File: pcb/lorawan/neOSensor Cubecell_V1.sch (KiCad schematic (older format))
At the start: 22 parts, among them J1 Conn_01x05, J2 Conn_01x05, J3 Conn_01x04, J5 Conn_01x05, J6 Conn_01x04, J7 ATECC508A, SW1 G71Y, U1 HTCC-AB01, U2 HC-SR01, U3 OLED1.3_I2C

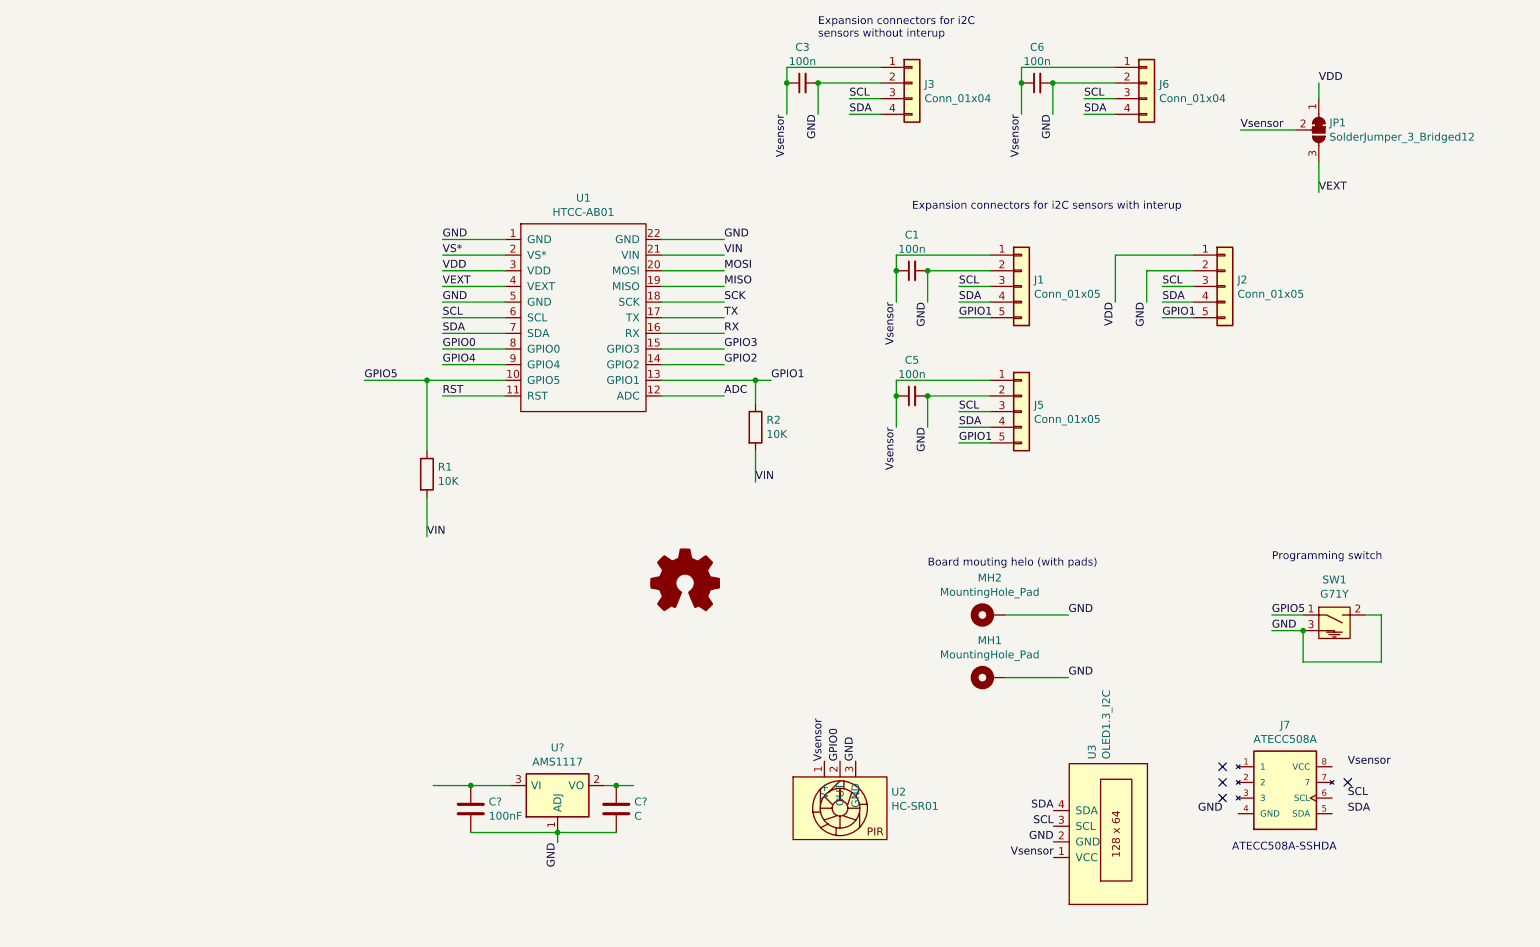
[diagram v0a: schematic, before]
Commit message: mise a jour des schema
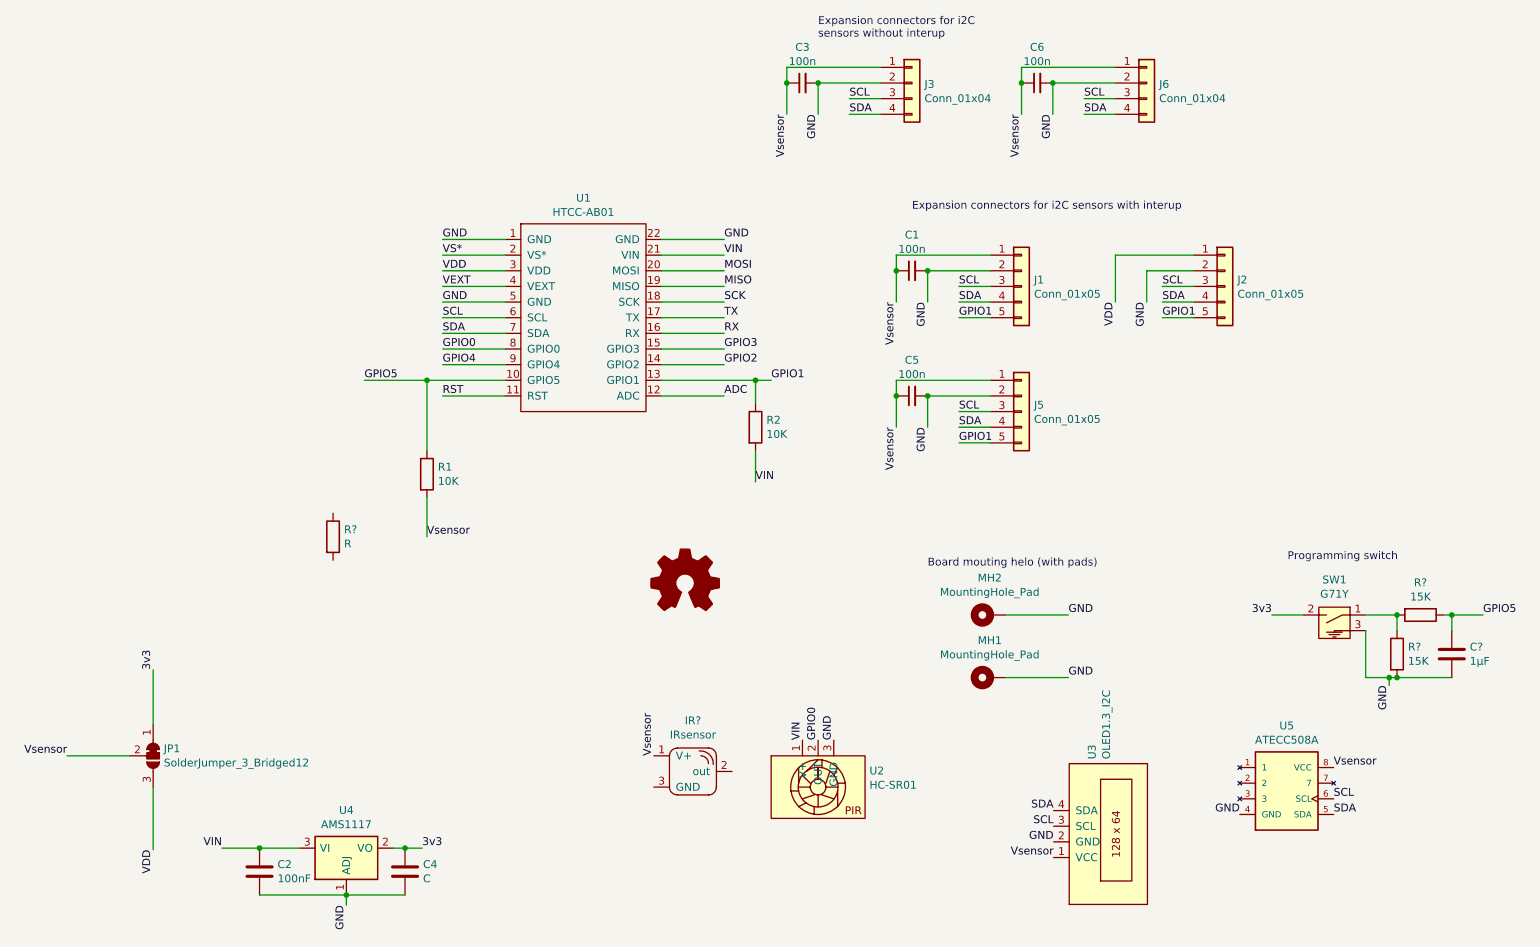
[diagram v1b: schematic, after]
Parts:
- removed J7: ATECC508A, neosensor_addon:ATECC508A, symbol neosensor_addon:ATECC508A
- removed SW1: G71Y, neosensor_addon:G71Y_µsw_smd, symbol neOSensor-Cubecell_V1-rescue:G71Y-neosensor_addon-neOSensor_Cubecell_V1-rescue
- removed U1: HTCC-AB01, HTCC-AB01:htcc-ab01, symbol neOSensor-Cubecell_V1-rescue:HTCC-AB01-htcc-ab01-neOSensor_Cubecell_V1-rescue
- added C?: 1µF, symbol Device:C
- added IR?: IRsensor, neosensor_addon:IRsensor_TH_and_smd, symbol neosensor_addon:IRsensor
- added R? (x2): 15K, symbol Device:R
- added R?: R, symbol Device:R
- added SW1: G71Y, neosensor_addon:G71Y_µsw_smd, symbol neosensor_addon:G71Y
- added U1: HTCC-AB01, neosensor_addon:HTCC-AB01, symbol neosensor_addon:HTCC-AB01
- added U5: ATECC508A, neosensor_addon:SOIC-8_3.9x5.4mm_P1.27mm_HandSolder, symbol neosensor_addon:ATECC508A
- C2, C4: renamed from C?; footprint (none) -> Capacitor_SMD:C_0805_2012Metric_Pad1.15x1.40mm_HandSolder
- gave numbers to parts that had none: 1
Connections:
- net ADC: now also U1.12 (ADC)
- net GND: now also C?.2, R?.2, SW1.3, U1.1 (GND), U1.22 (GND), U1.5 (GND), U5.4 (GND)
- net GPIO0: now also U1.8 (GPIO0)
- net GPIO1: now also U1.13 (GPIO1)
- net GPIO2: now also U1.14 (GPIO2)
- net GPIO3: now also U1.15 (GPIO3)
- net GPIO4: now also U1.9 (GPIO4)
- net GPIO5: now also C?.1, R?.1, U1.10 (GPIO5)
- net MISO: now also U1.19 (MISO)
- net MOSI: now also U1.20 (MOSI)
- net RST: now also U1.11 (RST)
- net RX: now also U1.16 (RX)
- net SCK: now also U1.18 (SCK)
- net SCL: now also U1.6 (SCL), U5.6 (SCL)
- net SDA: now also U1.7 (SDA), U5.5 (SDA)
- net TX: now also U1.17 (TX)
- net VDD: now also JP1.3 (B), U1.3 (VDD); no longer JP1.1 (A)
- net VEXT: now also U1.4 (VEXT); no longer JP1.3 (B)
- net VIN: now also C2.1, U2.1 (V+), U4.3 (VI), U1.21 (VIN); no longer R1.2
- net VS*: now also U1.2 (VS*)
- net Vsensor: now also R1.2, IR?.1 (V+), U5.8 (VCC); no longer U2.1 (V+)
- net 3v3: now reaches C4.1, U4.2 (VO)
- net 3v3: now also JP1.1 (A), SW1.2
- new net: R?.1, R?.2, SW1.1
- no-connect marks 4 -> 0
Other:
- note removed: "ATECC508A-SSHDA"
- moved on the sheet: C2, C4, JP1, U2, U4
